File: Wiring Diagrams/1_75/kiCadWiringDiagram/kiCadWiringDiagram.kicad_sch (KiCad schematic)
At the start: 28 parts, among them J1 ESP32, J12 Speaker Connector, J2 Encoder Connector, J3 LED Connector, J4 Motor Connector, J5 12v Input 1, J6 12v Input 2, U1 LM2596S-5, U2 MC34063AD, U3 MMC5603NJ, U4 TMC6300-LA, U5 MCP23017_ML

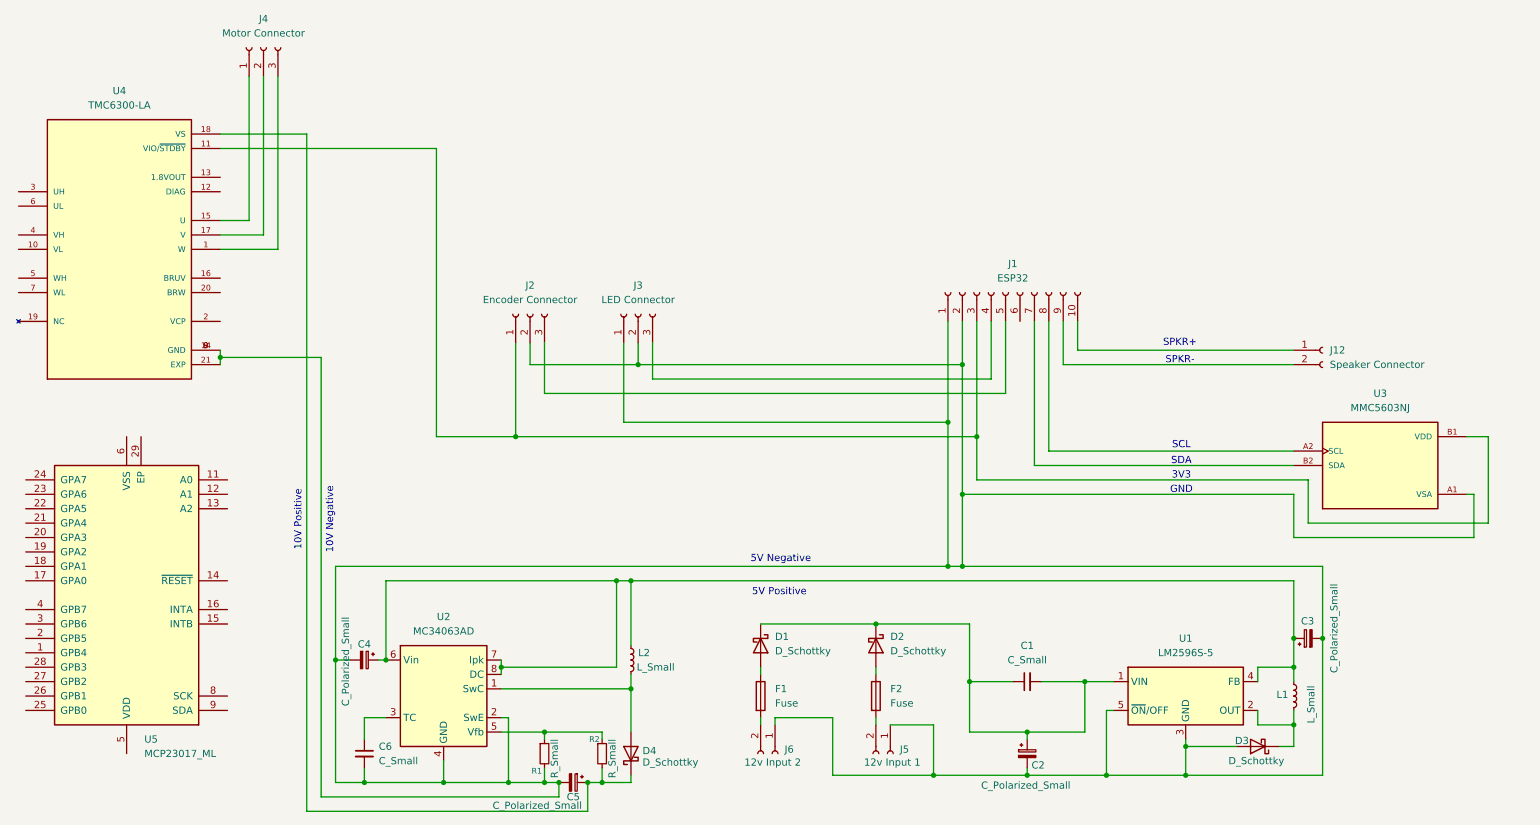
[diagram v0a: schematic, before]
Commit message: Schematic now done I think
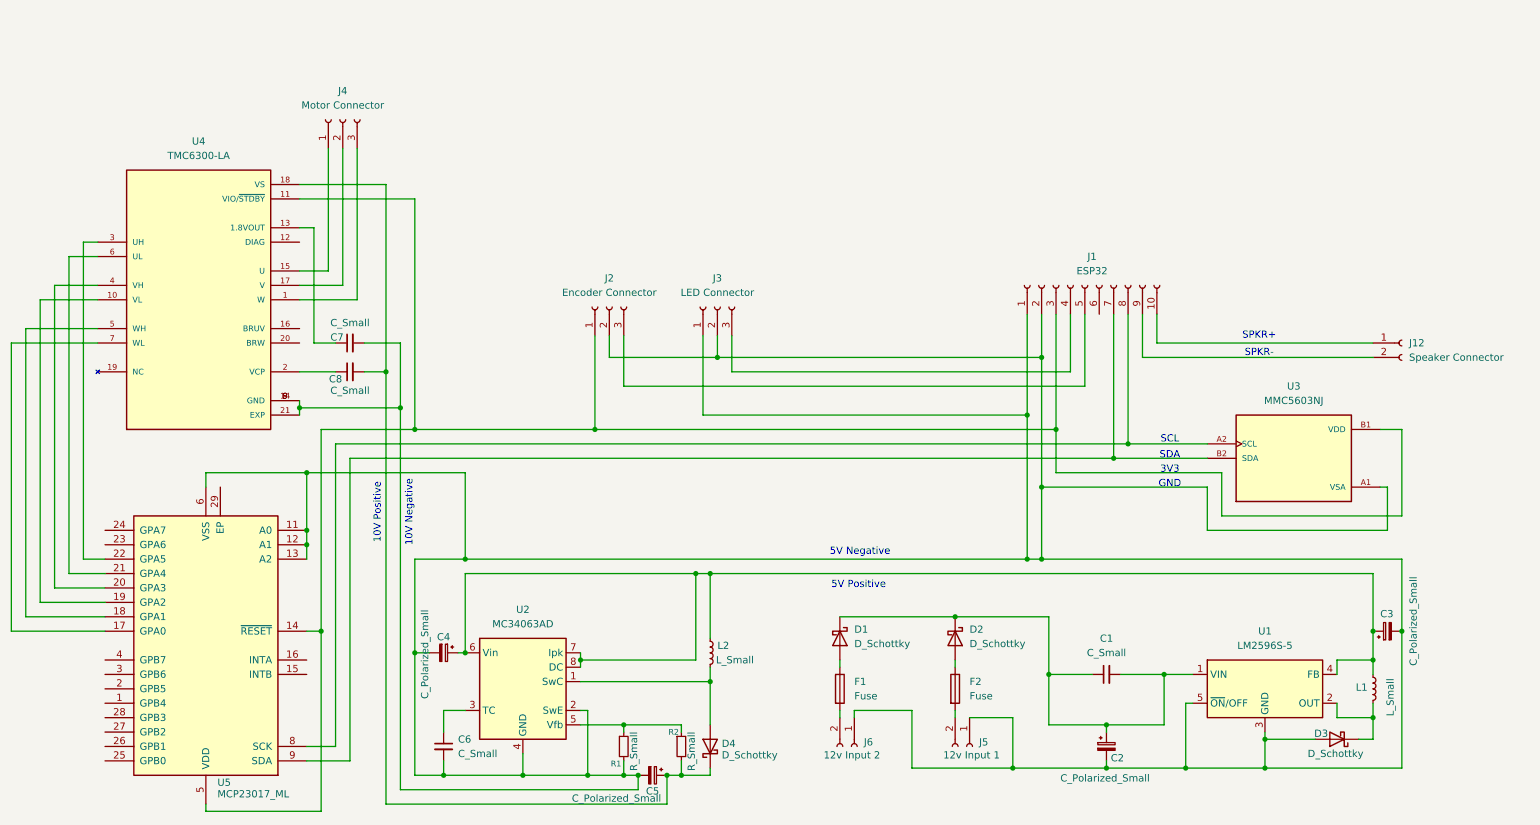
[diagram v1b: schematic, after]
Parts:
- added C7, C8: C_Small, symbol Device:C_Small
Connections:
- net at C2.2, C3.2, C4.2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: now also U5.11 (A0), U5.12 (A1), U5.13 (A2), U5.6 (VSS), C7.2
- net at J1.3 (Pin_3), J2.1 (Pin_1), U3.B1 (VDD)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: now also U5.14 (~{RESET}), U5.5 (VDD)
- net at J1.7 (Pin_7), U3.B2 (SDA): now also U5.9 (SDA)
- net at J1.8 (Pin_8), U3.A2 (SCL): now also U5.8 (SCK)
- net at U5.17 (GPA0): now also U4.7 (WL)
- net at U5.18 (GPA1): now also U4.5 (WH)
- net at U5.19 (GPA2): now also U4.10 (VL)
- net at U5.20 (GPA3): now also U4.4 (VH)
- net at U5.21 (GPA4): now also U4.6 (UL)
- net at U5.22 (GPA5): now also U4.3 (UH)
- net at U4.13 (1.8VOUT): now also C7.1
- net at C5.1, D4.1 (K), R2.2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: now also C8.2
- net at U4.2 (VCP): now also C8.1
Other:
- moved on the sheet: C1, C2, C3, C4, C5, C6, D1, D2, D3, D4, F1, F2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
